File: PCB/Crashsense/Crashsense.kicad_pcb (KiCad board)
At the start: 4 copper layers, 77.5 x 47.5 mm, 49 parts, among them J1 u-blox NEO-M8N, J2 Micro_SD_Card_Det1, J3 BATTERY_CONNECTOR, J4 Debug_pins, J5 Coincell_BAT, P1 USB_C_Plug_USB2.0, SW1 SW_Push, SW2 SW_Push, U1 ESP32-S3-WROOM-1, U2 ADXL377, U3 BMM150, U4 DS3231M, U5 BMI270, U6 TP4056-42-ESOP8, U7 ME6211C10M5

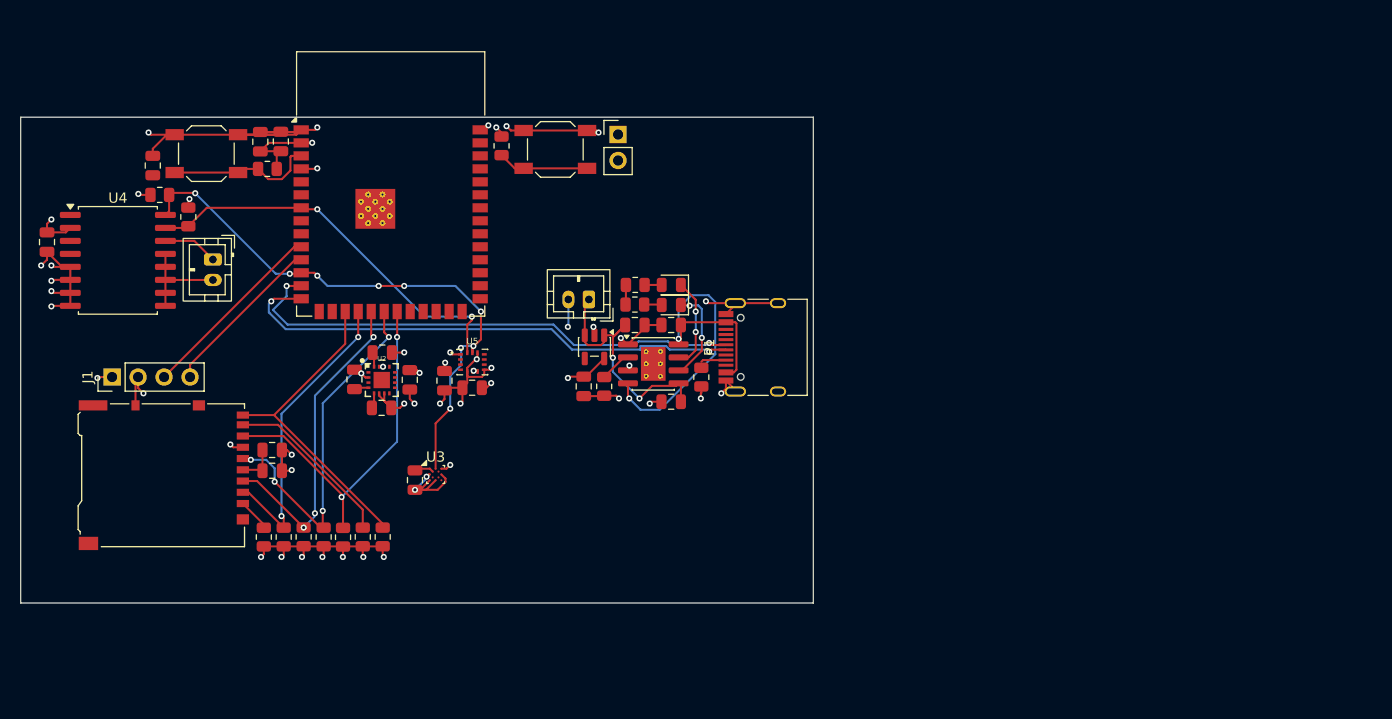
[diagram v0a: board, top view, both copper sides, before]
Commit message: PCb rerouting started and journalled for today
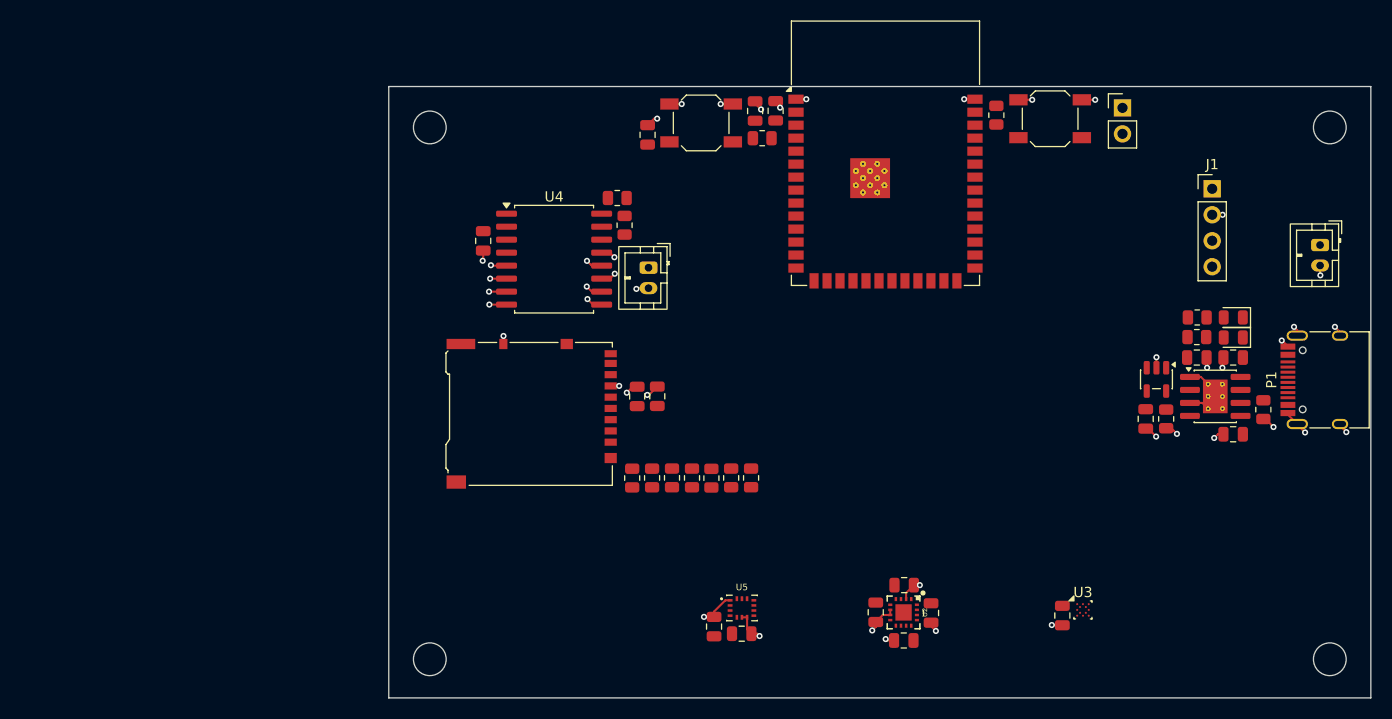
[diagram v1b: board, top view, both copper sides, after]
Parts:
- added REF**: MountingHole_3.2mm_M3, MountingHole:MountingHole_3.2mm_M3, F.Cu at (151.0, 132.5)
- added REF**: MountingHole_3.2mm_M3, MountingHole:MountingHole_3.2mm_M3, F.Cu at (239.0, 132.5)
- added REF**: MountingHole_3.2mm_M3, MountingHole:MountingHole_3.2mm_M3, F.Cu at (239.0, 80.5)
- added REF**: MountingHole_3.2mm_M3, MountingHole:MountingHole_3.2mm_M3, F.Cu at (151.0, 80.5)
- moved J1 109.1 mm to (227.5, 86.5), turned to 0 degrees
- moved J3 71.7 mm to (238.1, 92.0), turned to -90 degrees
- moved C14 64.7 mm to (212.8, 128.2)
- moved U3 64.7 mm to (214.9, 127.7)
- moved C10 59.4 mm to (200.0, 128.0), turned to -90 degrees
- moved C9 57.4 mm to (197.4, 125.3), turned to 0 degrees
- moved U2 55.9 mm to (197.3, 127.9), turned to -90 degrees
- moved C1 55.0 mm to (229.6, 103.0)
- moved C2 55.0 mm to (229.6, 110.5)
- moved U6 55.0 mm to (227.8, 106.8)
- moved U7 55.0 mm to (222.1, 105.1)
- moved C3 55.0 mm to (226.0, 103.0)
- moved C4 55.0 mm to (221.0, 109.0)
- moved D1 55.0 mm to (229.6, 101.0)
- moved D2 55.0 mm to (229.6, 99.1)
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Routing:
- net 3V3: track 62.7 -> 0.00 mm, vias 21 -> 0
- net GND: track 127.1 -> 66.7 mm, vias 33 -> 45
- net I2C_SCL: track 56.8 -> 0.00 mm, vias 9 -> 0
- net USB_D+: track 51.1 -> 0.00 mm, vias 2 -> 0
- net USB_D-: track 50.5 -> 0.00 mm, vias 2 -> 0
- net +5V_USB: track 41.2 -> 0.00 mm, vias 2 -> 0
- net I2C_SDA: track 38.9 -> 0.00 mm, vias 2 -> 0
- net SD_MISO: track 35.7 -> 0.00 mm, vias 2 -> 0
- net SD_SCK: track 35.5 -> 0.00 mm, vias 4 -> 0
- net SD_MOSI: track 31.9 -> 0.00 mm, vias 3 -> 0
- net SD_DET: track 31.5 -> 0.00 mm
- net SD_CS: track 29.8 -> 0.00 mm, vias 2 -> 0
- net VBAT: track 24.7 -> 0.00 mm, vias 2 -> 0
- net GPS_RX: track 18.7 -> 0.00 mm
- net DAT1: track 16.9 -> 0.00 mm
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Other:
- board size 77.5 x 47.5 mm -> 96 x 59.8 mm
